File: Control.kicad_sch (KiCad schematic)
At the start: 57 parts, among them J10 USB_C_Receptacle_USB2.0_16P, J8 Debug, J9 Magi Connector, Q1 DMN32D2LFB4, Q2 DMN32D2LFB4, Q3 DMN32D2LFB4, Q4 DMN32D2LFB4, Q5 DMN32D2LFB4, T1 GA021G00, T2 GA021G00, T3 GA021G00, T4 GA021G00, U16 TPS259474A, U17 W25Q128JVS, U18 RP2040, U19 TVS2200DRV, U20 ESD122DMYR, U21 ESD122DMYR, U22 TPD4EUSB30, U23 TPD4EUSB30, Y5 ABM8-272-T3

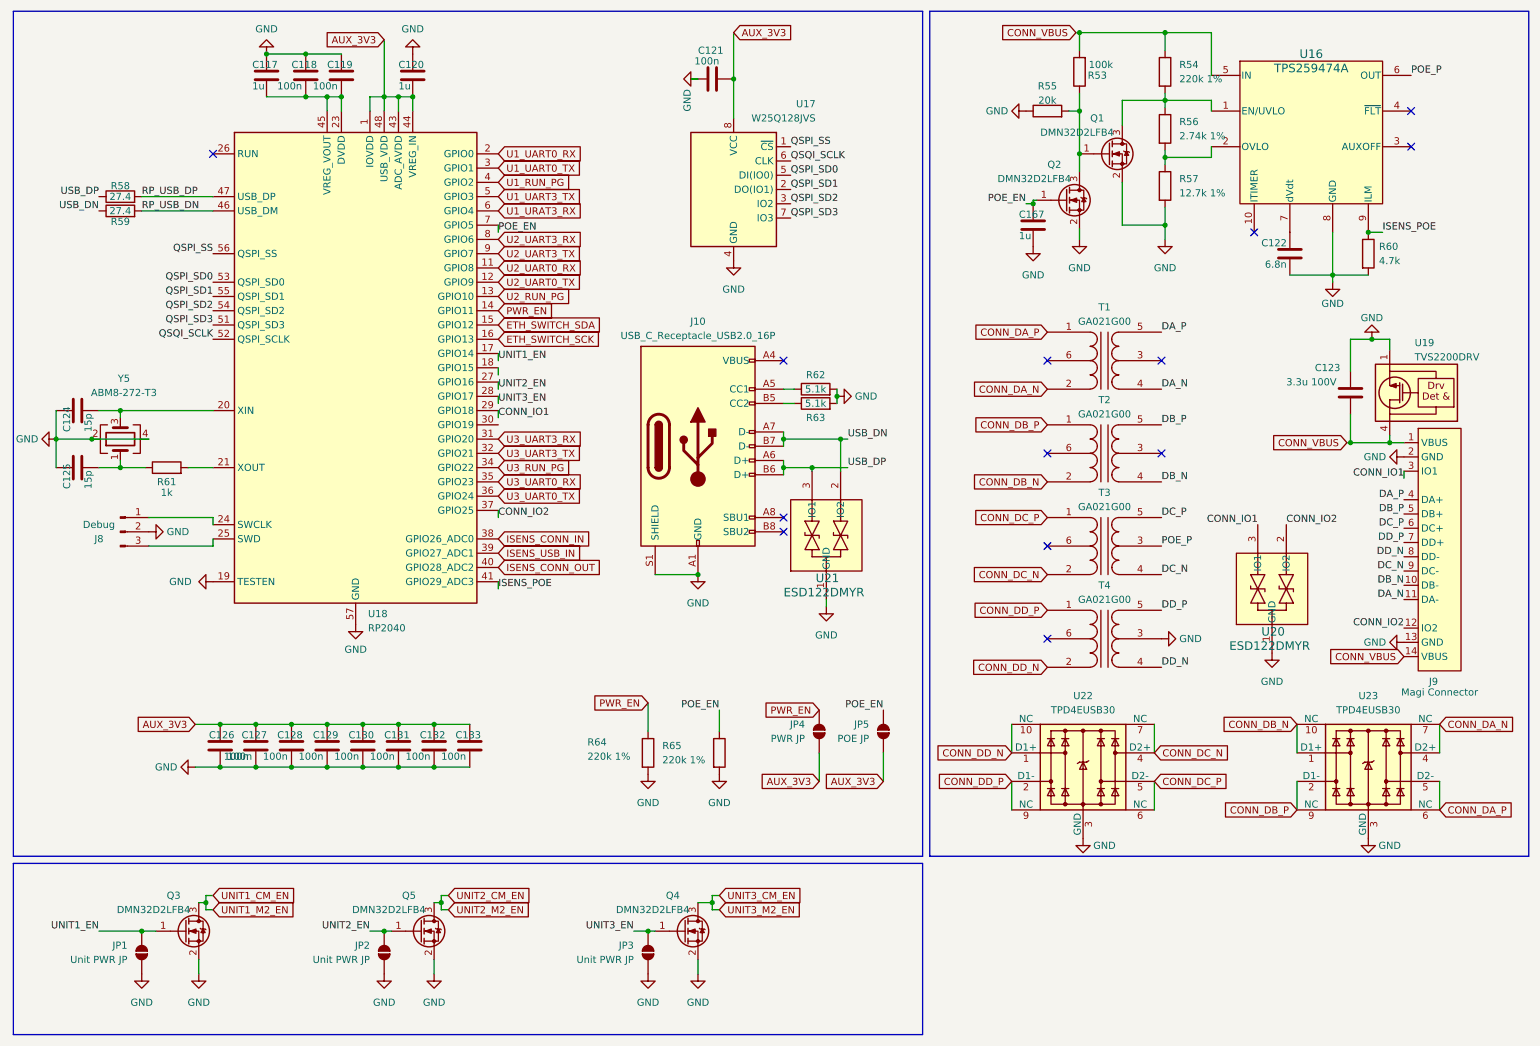
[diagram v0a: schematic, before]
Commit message: Magi v2.0
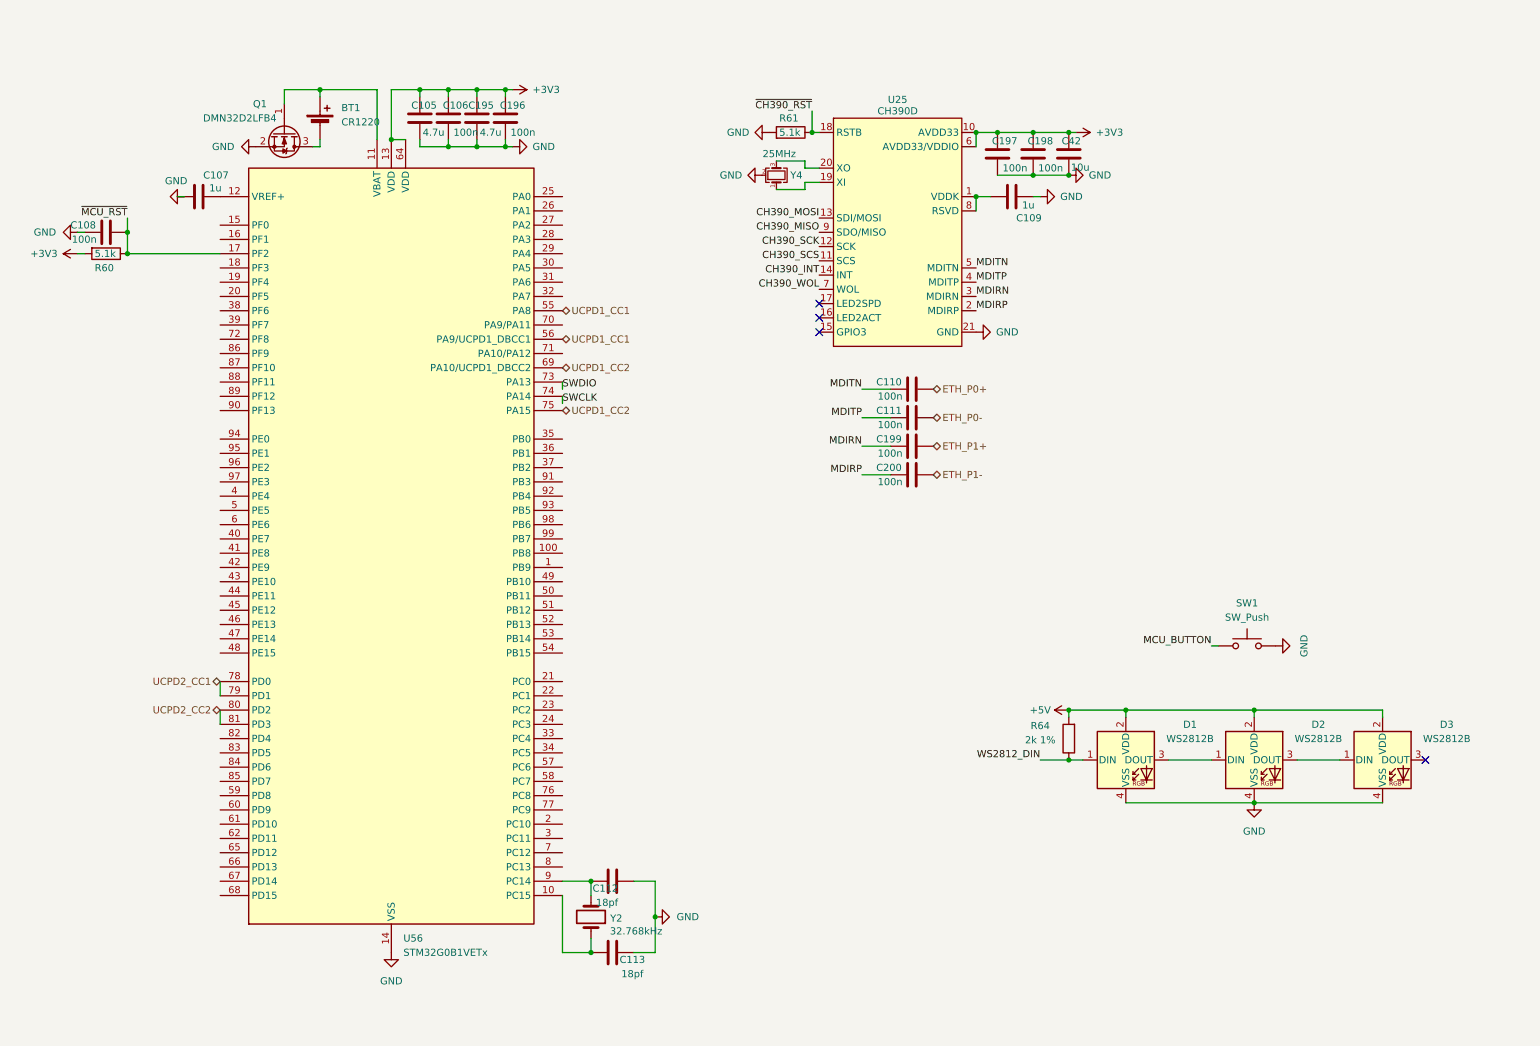
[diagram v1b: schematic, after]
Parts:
- removed C117, C120, C167: 1u, Capacitor_SMD:C_0402_1005Metric, symbol Device:C
- removed C118, C119, C121, C126, C127, C128, C129, C130, C131, C132, C133: 100n, Capacitor_SMD:C_0402_1005Metric, symbol Device:C
- removed C122: 6.8n, Capacitor_SMD:C_0603_1608Metric, symbol Device:C
- removed C123: 3.3u 100V, Capacitor_SMD:C_1210_3225Metric, symbol Device:C
- removed C124, C125: 15p, Capacitor_SMD:C_0402_1005Metric, symbol Device:C
- removed J10: USB_C_Receptacle_USB2.0_16P, Magi:USB-C-SMD_TYPEC-304J-BCP16, symbol Magi:USB_C_Receptacle_USB2.0_16P
- removed J8: Debug, Connector_JST:JST_SH_BM03B-SRSS-TB_1x03-1MP_P1.00mm_Vertical, symbol Connector:Conn_01x03_Pin
- removed J9: Magi Connector, Magi:HDR-SMD_14P-P2.54-H-F-L11.5, symbol Magi:Magi_Connector
- removed JP1, JP2, JP3: Unit PWR JP, Jumper:SolderJumper-2_P1.3mm_Open_TrianglePad1.0x1.5mm, symbol Jumper:SolderJumper_2_Open
- removed JP4: PWR JP, Jumper:SolderJumper-2_P1.3mm_Open_TrianglePad1.0x1.5mm, symbol Jumper:SolderJumper_2_Open
- removed JP5: POE JP, Jumper:SolderJumper-2_P1.3mm_Open_TrianglePad1.0x1.5mm, symbol Jumper:SolderJumper_2_Open
- removed Q2, Q3, Q4, Q5: DMN32D2LFB4, Package_DFN_QFN:Diodes_DFN1006-3, symbol Device:Q_NMOS_GSD
- removed R53: 100k, Resistor_SMD:R_0402_1005Metric, symbol Device:R
- removed R54, R65: 220k 1%, Resistor_SMD:R_0402_1005Metric, symbol Device:R
- removed R55: 20k, Resistor_SMD:R_0402_1005Metric, symbol Device:R
- removed R56: 2.74k 1%, Resistor_SMD:R_0402_1005Metric, symbol Device:R
- removed R57: 12.7k 1%, Resistor_SMD:R_0402_1005Metric, symbol Device:R
- removed R58, R59: 27.4, Resistor_SMD:R_0402_1005Metric, symbol Device:R
- removed R62, R63: 5.1k, Resistor_SMD:R_0402_1005Metric, symbol Device:R
- removed T1, T2, T3, T4: GA021G00, Magi:FILTER-SMD_6P-L4.5-W3.4_GA021G00, symbol Magi:Transformer_SP_SS
- removed U16: TPS259474A, Magi:RPW0010A-MFG, symbol Magi:TPS259470ARPWR
- removed U17: W25Q128JVS, Package_SO:SOIC-8_5.23x5.23mm_P1.27mm, symbol Memory_Flash:W25Q128JVS
- removed U18: RP2040, Package_DFN_QFN:QFN-56-1EP_7x7mm_P0.4mm_EP3.2x3.2mm, symbol MCU_RaspberryPi:RP2040
- removed U19: TVS2200DRV, Package_SON:WSON-6-1EP_2x2mm_P0.65mm_EP1x1.6mm, symbol Power_Protection:TVS2200DRV
- removed U20, U21: ESD122DMYR, Magi:DMY0003A, symbol Magi:ESD122DMYR
- removed U22, U23: TPD4EUSB30, Magi:USON-10_2.5x1.0mm_P0.5mm, symbol Power_Protection:TPD4EUSB30
- removed Y5: ABM8-272-T3, Crystal:Crystal_SMD_3225-4Pin_3.2x2.5mm, symbol Device:Crystal_GND24
- added BT1: CR1220, Magi:BAT-SMD_MY-1220-03, symbol Device:Battery_Cell
- added C105, C195: 4.7u, Capacitor_SMD:C_0603_1608Metric, symbol Device:C
- added C106, C108, C110, C111, C196, C197, C198, C199, C200: 100n, Capacitor_SMD:C_0402_1005Metric, symbol Device:C
- added C107, C109: 1u, Capacitor_SMD:C_0603_1608Metric, symbol Device:C
- added C112, C113: 18pf, Capacitor_SMD:C_0402_1005Metric, symbol Device:C
- added C42: 10u, Capacitor_SMD:C_0603_1608Metric, symbol Device:C
- added D1, D2, D3: WS2812B, Magi:LED-SMD_4P-L4.0-W1.7-R, symbol PiCard:WS2812C-4020
- added SW1: SW_Push, Magi:SW-SMD_L4.7-W3.5-P3.35-EH, symbol Switch:SW_Push
- added U25: CH390D, Package_DFN_QFN:QFN-20-1EP_3x3mm_P0.4mm_EP1.65x1.65mm, symbol Magi:CH390D
- added U56: STM32G0B1VETx, Package_QFP:LQFP-100_14x14mm_P0.5mm, symbol MCU_ST_STM32G0:STM32G0B1VETx
- added Y2: 32.768kHz, Crystal:Crystal_SMD_2012-2Pin_2.0x1.2mm, symbol Device:Crystal
- added Y4: 25MHz, Crystal:Crystal_SMD_2016-4Pin_2.0x1.6mm, symbol Device:Crystal_GND24_Small
- R60: value 4.7k -> 5.1k; LCSC C25900 -> C25905; MPN 0402WGF4701TCE -> 0402WGF5101TCE
- R61: value 1k -> 5.1k; LCSC C11702 -> C25905; MPN 0402WGF1001TCE -> 0402WGF5101TCE
- R64: value 220k 1% -> 2k 1%; LCSC C25767 -> C4109; MPN 0402WGF2203TCE -> 0402WGF2001TCE
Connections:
- net GND: now also R61.2, C105.2, C106.1, C107.1, C108.1, C109.2, C112.1, C113.1, C195.2, C196.1, C197.1, C198.1, C42.2, D1.4 (VSS), D2.4 (VSS), D3.4 (VSS), SW1.1, U25.21 (GND), U56.14 (VSS), U56.63 (VSS), Y4.2 (G), Y4.4 (G); no longer R60.2, R64.2
- net at Q1.1 (G): now also BT1.1 (+), U56.11 (VBAT)
- net at Q1.3 (D): now also BT1.2 (-)
- net ~{CH390_RST}: now reaches R61.1
- net ~{CH390_RST}: now also U25.18 (RSTB)
- net ISENS_POE renamed ~{MCU_RST}
- net ~{MCU_RST}: now also C108.2, U56.17 (PF2)
- net PWR_EN renamed WS2812_DIN
- net WS2812_DIN: now also D1.1 (DIN)
- new net: C107.2, U56.12 (VREF+)
- new net: C113.2, U56.10 (PC15), Y2.1
- new net: D2.3 (DOUT), D3.1 (DIN)
- new net: C109.1, U25.1 (VDDK), U25.8 (RSVD)
- new net: U25.19 (XI), Y4.1
- new net: U25.20 (XO), Y4.3
- new net: D1.3 (DOUT), D2.1 (DIN)
- new net: C112.2, U56.9 (PC14), Y2.2
- new net +3V3: C105.1, C106.2, C195.1, C196.2, C197.2, C198.2, C42.1, R60.2, U25.10 (AVDD33), U25.6 (AVDD33/VDDIO), U56.13 (VDD), U56.64 (VDD)
- new net +5V: D1.2 (VDD), D2.2 (VDD), D3.2 (VDD), R64.2
- new net CH390_INT: U25.14 (INT)
- new net CH390_MISO: U25.9 (SDO/MISO)
- new net CH390_MOSI: U25.13 (SDI/MOSI)
- new net CH390_SCK: U25.12 (SCK)
- new net CH390_SCS: U25.11 (SCS)
- new net CH390_WOL: U25.7 (WOL)
- new net ETH_P0+: C110.2
- new net ETH_P0-: C111.2
- new net ETH_P1+: C199.2
- new net ETH_P1-: C200.2
- new net MCU_BUTTON: SW1.2
- new net MDIRN: C199.1, U25.3 (MDIRN)
- new net MDIRP: C200.1, U25.2 (MDIRP)
- new net MDITN: C110.1, U25.5 (MDITN)
- new net MDITP: C111.1, U25.4 (MDITP)
- new net SWCLK: U56.74 (PA14)
- new net SWDIO: U56.73 (PA13)
- new net UCPD1_CC1: U56.55 (PA8), U56.56 (PA9/UCPD1_DBCC1)
- new net UCPD1_CC2: U56.69 (PA10/UCPD1_DBCC2), U56.75 (PA15)
- new net UCPD2_CC1: U56.78 (PD0), U56.79 (PD1)
- new net UCPD2_CC2: U56.80 (PD2), U56.81 (PD3)
- no-connect marks 13 -> 4
